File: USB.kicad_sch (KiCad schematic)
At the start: 55 parts, among them J1 USB_C_Receptacle_USB2.0, J2 USB_A, J3 USB_A, J4 USB_A, U5 NUP2202, U6 NUP2202, U7 NUP2202, U8 NUP2202, Y1 12MHz

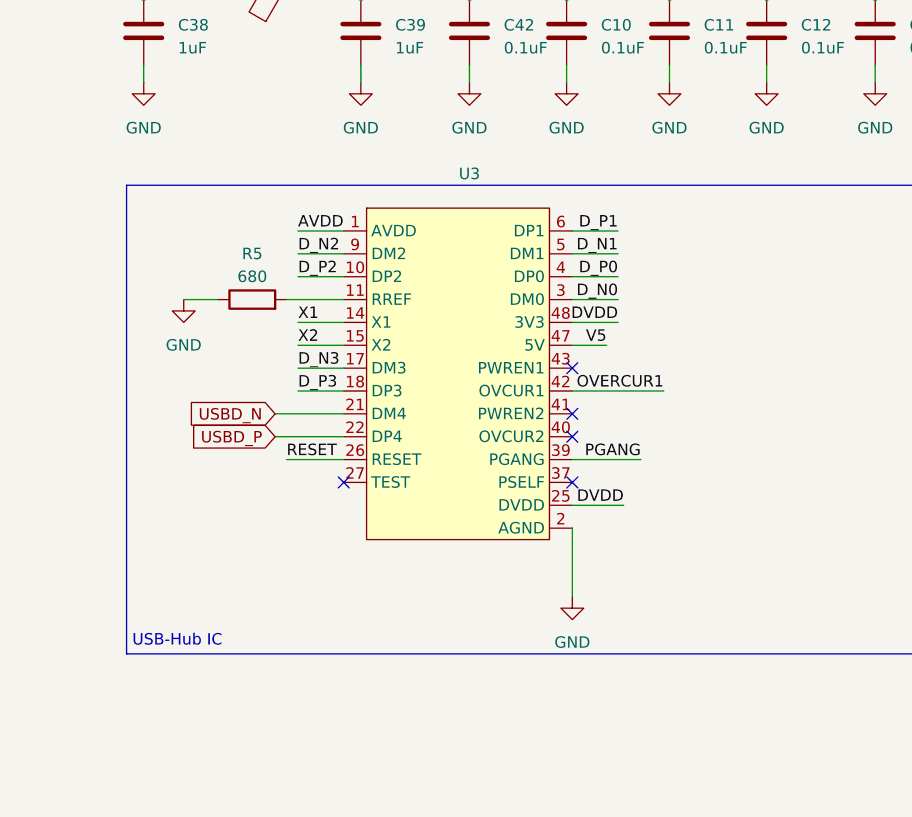
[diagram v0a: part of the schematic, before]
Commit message: Add files via upload
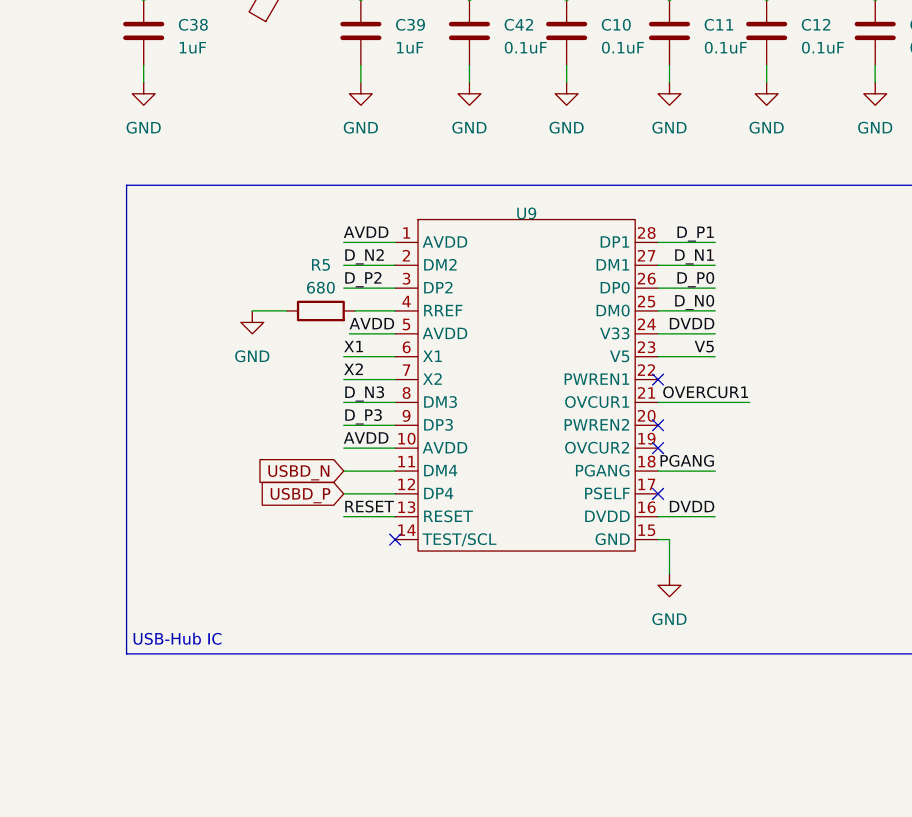
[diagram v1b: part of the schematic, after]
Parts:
- removed U3: ~, Package_QFP:LQFP-48_7x7mm_P0.5mm, symbol GL850G-HH:GL850G-HH
- added U9: ~, Package_SO:SSOP-28_5.3x10.2mm_P0.65mm, symbol GL850G-HH:GL850G-HH
- C22, C24, C26: footprint Capacitor_SMD:CP_Elec_6.3x7.7 -> Capacitor_SMD:C_1206_3216Metric_Pad1.33x1.80mm_HandSolder
- R5, R7: footprint Resistor_SMD:R_0805_2012Metric_Pad1.20x1.40mm_HandSolder -> Resistor_SMD:R_0603_1608Metric_Pad0.98x0.95mm_HandSolder
- TH1, TH2, TH4: footprint Fuse:Fuse_0805_2012Metric_Pad1.15x1.40mm_HandSolder -> Fuse:Fuse_0402_1005Metric_Pad0.77x0.64mm_HandSolder
- U5, U6, U7, U8: footprint Package_TO_SOT_SMD:TSOT-23-6 -> Package_TO_SOT_SMD:SOT-363_SC-70-6_Handsoldering
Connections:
- net +5V: now also U9.23 (V5)
- net AVDD: now also U9.1 (AVDD), U9.10 (AVDD), U9.5 (AVDD)
- net DVDD: now also U9.16 (DVDD), U9.24 (V33)
- net D_N0: now also U9.25 (DM0)
- net D_N1: now also U9.27 (DM1)
- net D_N2: now also U9.2 (DM2)
- net D_N3: now also U9.8 (DM3)
- net D_P0: now also U9.26 (DP0)
- net D_P1: now also U9.28 (DP1)
- net D_P2: now also U9.3 (DP2)
- net D_P3: now also U9.9 (DP3)
- net OVERCUR1: now also U9.21 (OVCUR1)
- net PGANG: now also U9.18 (PGANG)
- net RESET: now also U9.13 (RESET)
- net USBD_N: now also U9.11 (DM4)
- net USBD_P: now also U9.12 (DP4)
- net X1: now also U9.6 (X1)
- net X2: now also U9.7 (X2)
- net at R5.2: now also U9.4 (RREF)
- net AGND renamed GND
- net GND: now also U9.15 (GND)
